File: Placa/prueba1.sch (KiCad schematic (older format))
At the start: 51 parts, among them J1 JACK_2P, U1 MAX232_TID, U2 LM2937, U3 MAX874

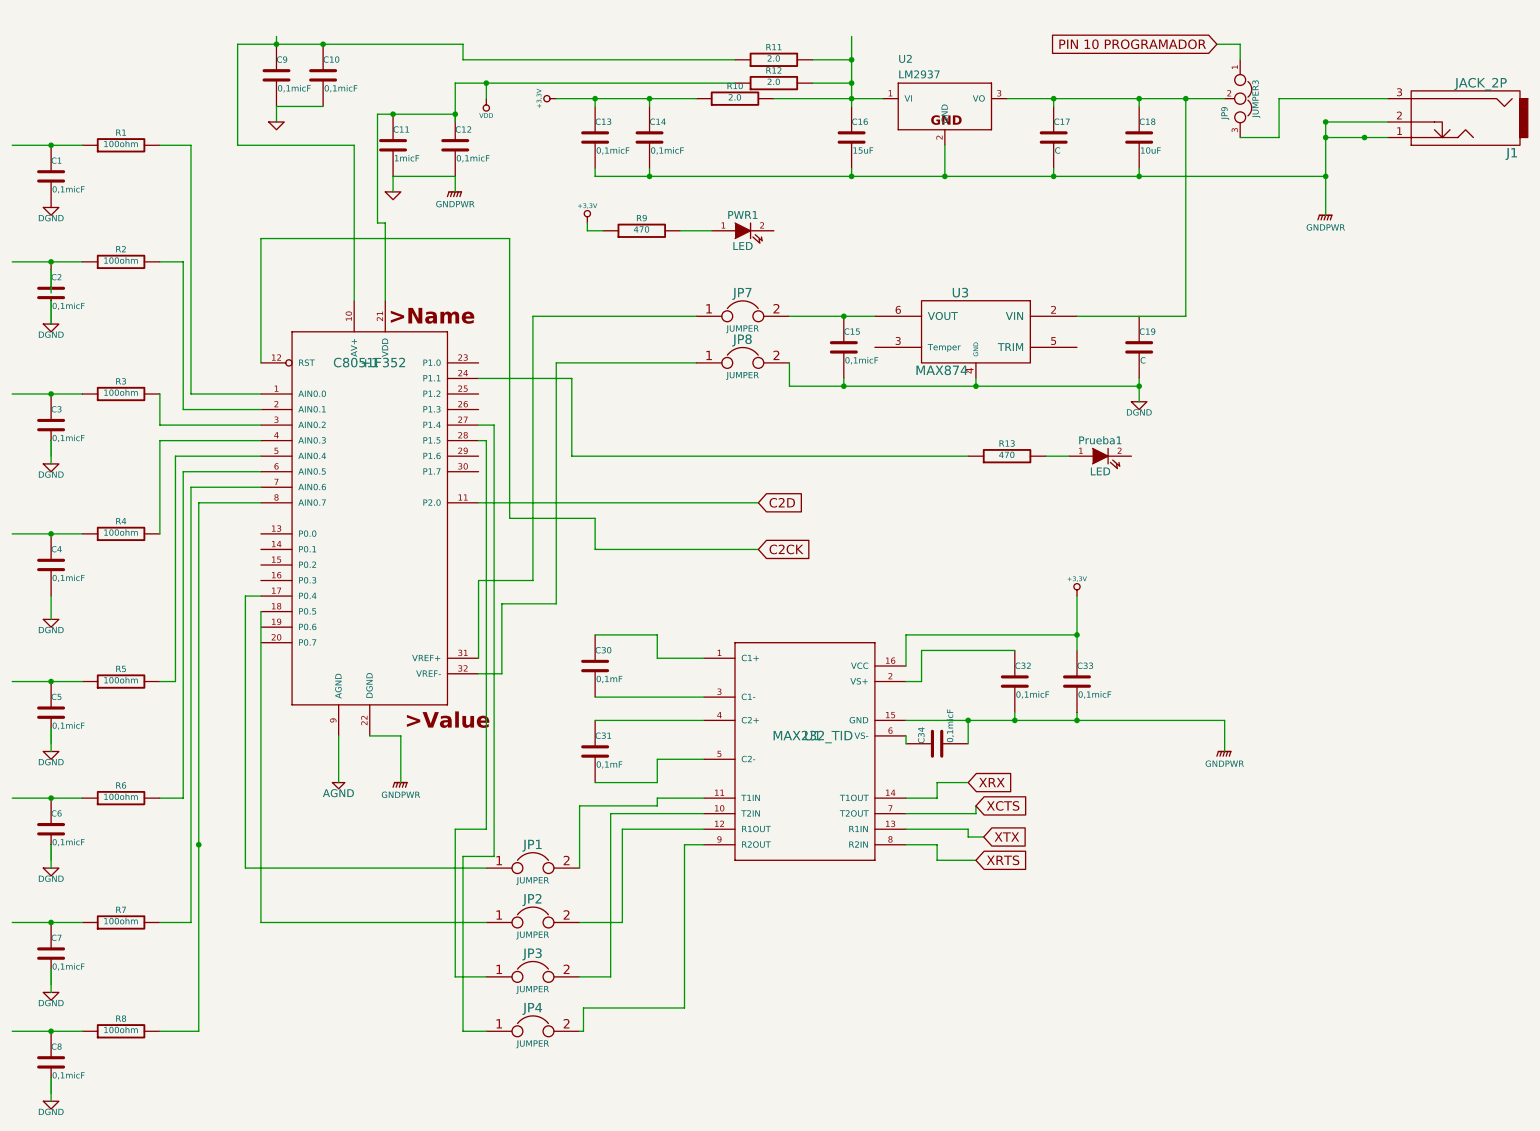
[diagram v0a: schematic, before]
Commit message: Commit Prueba Archivos Placa
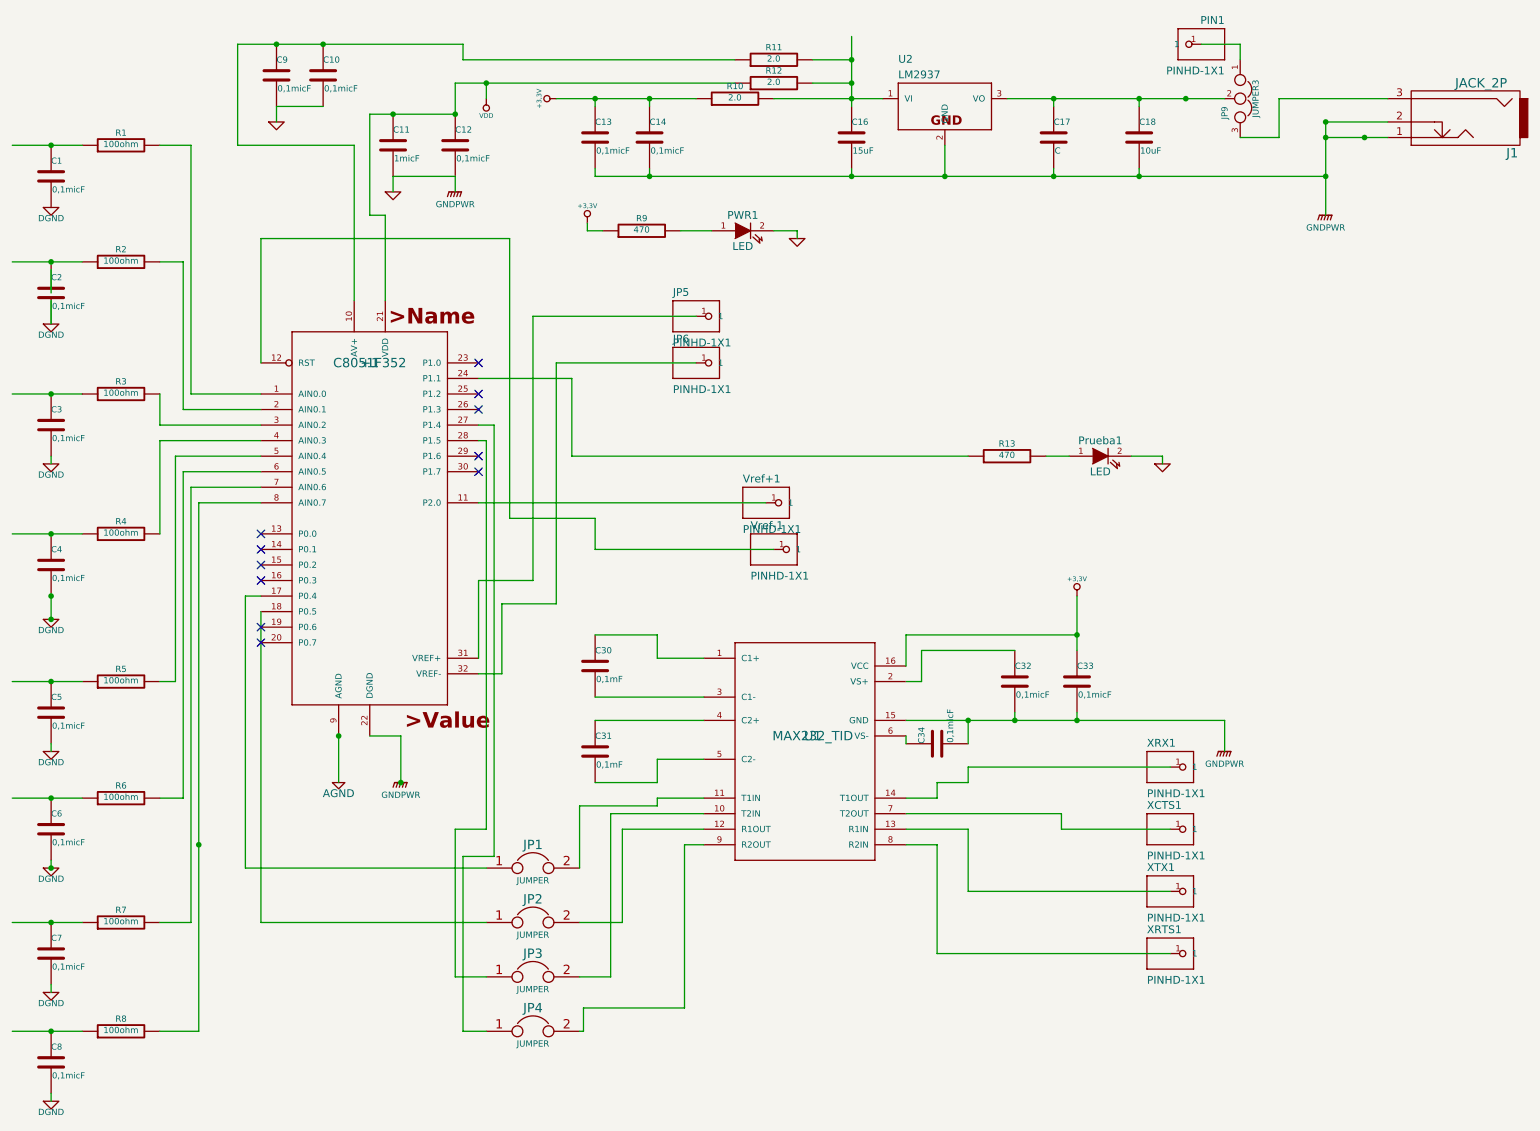
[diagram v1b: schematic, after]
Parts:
- removed C15: 0,1micF, ~, symbol C
- removed C19: C, ~, symbol C
- removed JP7, JP8: JUMPER, ~, symbol JUMPER
- removed U3: MAX874, ~, symbol MAX874
- added JP5, JP6, PIN1, Vref+1, Vref-1, XCTS1, XRTS1, XRX1, XTX1: PINHD-1X1, pinhead-1X01, symbol PINHD-1X1
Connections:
- net labels removed: C2CK, C2D, PIN 10 PROGRAMADOR, XCTS, XRTS, XRX, XTX
- wire segments 177 -> 175
- no-connect marks 0 -> 11

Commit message: Merge remote-tracking branch 'origin/master'
Conflicts:
	.gitignore
	Placa/prueba1.lst
	Source/fuentes/adc
	Source/fuentes/adc.#1
	Source/fuentes/adc.#2
	Source/fuentes/adc.#3
	Source/fuentes/adc.M51
	Source/fuentes/comunicacion.#1
	Source/fuentes/comunicacion.#3
	Source/fuentes/comunicacion.LST
	Source/fuentes/comunicacion.M51
	Source/fuentes/comunicacion.OBJ
	Source/fuentes/configurador.LST
	Source/fuentes/configurador.OBJ
	Source/fuentes/conversor.LST
	Source/fuentes/conversor.OBJ
	Source/fuentes/interfaz.LST
	Source/fuentes/interfaz.OBJ
	Source/fuentes/interrupciones.LST
	Source/fuentes/interrupciones.OBJ
	Source/fuentes/main.LST
	Source/fuentes/main.OBJ
	Source/fuentes/memoria.LST
	Source/fuentes/memoria.OBJ
	Source/test/test_comunicacion.LST
	Source/test/test_comunicacion.OBJ
	Source/test/test_global.LST
	Source/test/test_global.OBJ

commit onda
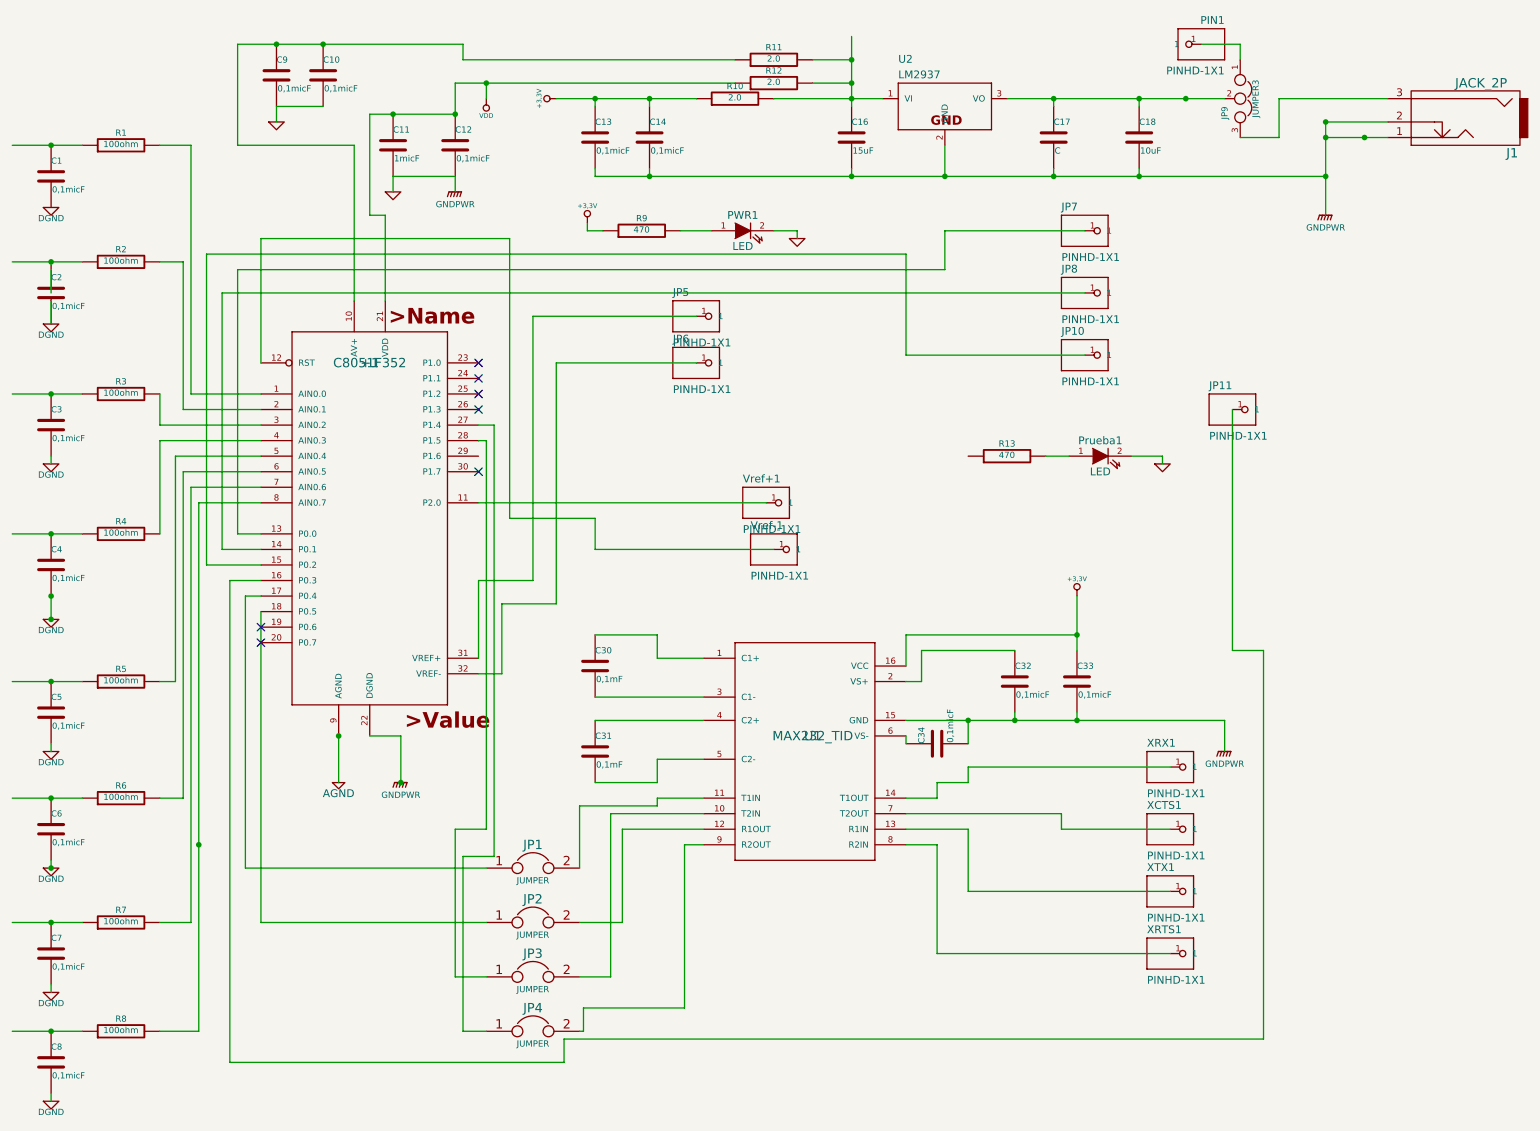
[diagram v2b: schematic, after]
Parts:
- added JP10, JP11, JP7, JP8: PINHD-1X1, pinhead-1X01, symbol PINHD-1X1
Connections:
- wire segments 175 -> 193
- no-connect marks 11 -> 7
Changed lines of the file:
@@
 Sheet 1 1
 Title ""
-Date "4 may 2015"
+Date "8 may 2015"
 Rev ""
 Comp ""
@@
 $EndDescr
 $Comp
-L AGND #PWR10
+L AGND #PWR01
 U 1 1 5524219B
 P 3100 5400
-F 0 "#PWR10" H 3100 5400 40  0001 C CNN
+F 0 "#PWR01" H 3100 5400 40  0001 C CNN
 F 1 "AGND" H 3100 5330 50  0000 C CNN
 F 2 "" H 3100 5400 60  0000 C CNN
@@
 $EndComp
 $Comp
-L DGND #PWR3
+L DGND #PWR02
 U 1 1 552424EC
 P 1250 3350
-F 0 "#PWR3" H 1250 3350 40  0001 C CNN
+F 0 "#PWR02" H 1250 3350 40  0001 C CNN
 F 1 "DGND" H 1250 3280 40  0000 C CNN
 F 2 "" H 1250 3350 60  0000 C CNN
@@
 $EndComp
 $Comp
-L DGND #PWR2
+L DGND #PWR03
 U 1 1 5524256F
 P 1250 2450
-F 0 "#PWR2" H 1250 2450 40  0001 C CNN
+F 0 "#PWR03" H 1250 2450 40  0001 C CNN
 F 1 "DGND" H 1250 2380 40  0000 C CNN
 F 2 "" H 1250 2450 60  0000 C CNN
@@
 $EndComp
 $Comp
-L DGND #PWR1
+L DGND #PWR04
 U 1 1 55242585
 P 1250 1700
-F 0 "#PWR1" H 1250 1700 40  0001 C CNN
+F 0 "#PWR04" H 1250 1700 40  0001 C CNN
 F 1 "DGND" H 1250 1630 40  0000 C CNN
 F 2 "" H 1250 1700 60  0000 C CNN
@@
 $EndComp
 $Comp
-L DGND #PWR4
+L DGND #PWR05
 U 1 1 5524259B
 P 1250 4350
-F 0 "#PWR4" H 1250 4350 40  0001 C CNN
+F 0 "#PWR05" H 1250 4350 40  0001 C CNN
 F 1 "DGND" H 1250 4280 40  0000 C CNN
 F 2 "" H 1250 4350 60  0000 C CNN
@@
 $EndComp
 $Comp
-L DGND #PWR5
+L DGND #PWR06
 U 1 1 552425BD
 P 1250 5200
-F 0 "#PWR5" H 1250 5200 40  0001 C CNN
+F 0 "#PWR06" H 1250 5200 40  0001 C CNN
 F 1 "DGND" H 1250 5130 40  0000 C CNN
 F 2 "" H 1250 5200 60  0000 C CNN
@@
 $EndComp
 $Comp
-L DGND #PWR6
+L DGND #PWR07
 U 1 1 552425D3
 P 1250 5950
-F 0 "#PWR6" H 1250 5950 40  0001 C CNN
+F 0 "#PWR07" H 1250 5950 40  0001 C CNN
 F 1 "DGND" H 1250 5880 40  0000 C CNN
 F 2 "" H 1250 5950 60  0000 C CNN
@@
 $EndComp
 $Comp
-L DGND #PWR7
+L DGND #PWR08
 U 1 1 552426C6
 P 1250 6750
-F 0 "#PWR7" H 1250 6750 40  0001 C CNN
+F 0 "#PWR08" H 1250 6750 40  0001 C CNN
 F 1 "DGND" H 1250 6680 40  0000 C CNN
 F 2 "" H 1250 6750 60  0000 C CNN
@@
 $EndComp
 $Comp
-L DGND #PWR8
+L DGND #PWR09
 U 1 1 552426DB
 P 1250 7450
-F 0 "#PWR8" H 1250 7450 40  0001 C CNN
+F 0 "#PWR09" H 1250 7450 40  0001 C CNN
 F 1 "DGND" H 1250 7380 40  0000 C CNN
 F 2 "" H 1250 7450 60  0000 C CNN
@@
 $EndComp
 $Comp
-L GNDPWR #PWR21
+L GNDPWR #PWR010
 U 1 1 552C3CA0
 P 9450 1750
-F 0 "#PWR21" H 9450 1800 40  0001 C CNN
+F 0 "#PWR010" H 9450 1800 40  0001 C CNN
 F 1 "GNDPWR" H 9450 1670 40  0000 C CNN
 F 2 "" H 9450 1750 60  0000 C CNN
@@
 $EndComp
 $Comp
-L +3,3V #PWR15
+L +3,3V #PWR011
 U 1 1 552C5A6E
 P 4500 1000
-F 0 "#PWR15" H 4500 960 30  0001 C CNN
+F 0 "#PWR011" H 4500 960 30  0001 C CNN
 F 1 "+3,3V" H 4500 1110 30  0000 C CNN
 F 2 "" H 4500 1000 60  0000 C CNN
@@
 $EndComp
 $Comp
-L GNDPWR #PWR13
+L GNDPWR #PWR012
 U 1 1 552C5FBB
 P 3850 1600
-F 0 "#PWR13" H 3850 1650 40  0001 C CNN
+F 0 "#PWR012" H 3850 1650 40  0001 C CNN
 F 1 "GNDPWR" H 3850 1520 40  0000 C CNN
 F 2 "" H 3850 1600 60  0000 C CNN
@@
 $EndComp
 $Comp
-L GND #PWR11
+L GND #PWR013
 U 1 1 552C5FCA
 P 3450 1600
-F 0 "#PWR11" H 3450 1600 30  0001 C CNN
+F 0 "#PWR013" H 3450 1600 30  0001 C CNN
 F 1 "GND" H 3450 1530 30  0001 C CNN
 F 2 "" H 3450 1600 60  0000 C CNN
@@
 $EndComp
 $Comp
-L GND #PWR9
+L GND #PWR014
 U 1 1 552C6618
 P 2700 1150
-F 0 "#PWR9" H 2700 1150 30  0001 C CNN
+F 0 "#PWR014" H 2700 1150 30  0001 C CNN
 F 1 "GND" H 2700 1080 30  0001 C CNN
 F 2 "" H 2700 1150 60  0000 C CNN
@@
 	3500 5100 3500 5400
 $Comp
-L GNDPWR #PWR12
+L GNDPWR #PWR015
 U 1 1 552C76EE
 P 3500 5400
-F 0 "#PWR12" H 3500 5450 40  0001 C CNN
+F 0 "#PWR015" H 3500 5450 40  0001 C CNN
 F 1 "GNDPWR" H 3500 5320 40  0000 C CNN
 F 2 "" H 3500 5400 60  0000 C CNN
@@
 $EndComp
 $Comp
-L GNDPWR #PWR20
+L GNDPWR #PWR016
 U 1 1 552C76FD
 P 8800 5200
-F 0 "#PWR20" H 8800 5250 40  0001 C CNN
+F 0 "#PWR016" H 8800 5250 40  0001 C CNN
 F 1 "GNDPWR" H 8800 5120 40  0000 C CNN
 F 2 "" H 8800 5200 60  0000 C CNN
@@
 $EndComp
 $Comp
-L +3,3V #PWR18
+L +3,3V #PWR017
 U 1 1 552C770C
 P 7850 4200
-F 0 "#PWR18" H 7850 4160 30  0001 C CNN
+F 0 "#PWR017" H 7850 4160 30  0001 C CNN
 F 1 "+3,3V" H 7850 4310 30  0000 C CNN
 F 2 "" H 7850 4200 60  0000 C CNN
@@
 Wire Wire Line
 	1250 4200 1250 4350
-Wire Wire Line
-	4600 2800 4600 3300
-Wire Wire Line
-	4000 2800 4600 2800
-Wire Wire Line
-	4600 3300 7150 3300
-$Comp
-L +3,3V #PWR16
+$Comp
+L +3,3V #PWR018
 U 1 1 55313060
 P 4700 1800
-F 0 "#PWR16" H 4700 1760 30  0001 C CNN
+F 0 "#PWR018" H 4700 1760 30  0001 C CNN
 F 1 "+3,3V" H 4700 1910 30  0000 C CNN
 F 2 "" H 4700 1800 60  0000 C CNN
@@
 NoConn ~ 2600 4400
 NoConn ~ 2600 4500
-NoConn ~ 2600 4100
-NoConn ~ 2600 4000
-NoConn ~ 2600 3900
-NoConn ~ 2600 3800
-NoConn ~ 4000 2700
-NoConn ~ 4000 2900
-NoConn ~ 4000 3000
-NoConn ~ 4000 3300
 NoConn ~ 4000 3400
 Connection ~ 1250 4350
@@
 	3100 5400 3100 5100
 $Comp
-L GND #PWR17
+L GND #PWR019
 U 1 1 553FFE63
 P 6050 1900
-F 0 "#PWR17" H 6050 1900 30  0001 C CNN
+F 0 "#PWR019" H 6050 1900 30  0001 C CNN
 F 1 "GND" H 6050 1830 30  0001 C CNN
 F 2 "" H 6050 1900 60  0000 C CNN
@@
 	6050 1850 6050 1900
 $Comp
-L GND #PWR19
+L GND #PWR020
 U 1 1 553FFF60
 P 8400 3350
-F 0 "#PWR19" H 8400 3350 30  0001 C CNN
+F 0 "#PWR020" H 8400 3350 30  0001 C CNN
 F 1 "GND" H 8400 3280 30  0001 C CNN
 F 2 "" H 8400 3350 60  0000 C CNN
@@
 $EndComp
 $Comp
-L VDD #PWR14
+L VDD #PWR021
 U 1 1 552C5BF6
 P 4050 1000
-F 0 "#PWR14" H 4050 1100 30  0001 C CNN
+F 0 "#PWR021" H 4050 1100 30  0001 C CNN
 F 1 "VDD" H 4050 1110 30  0000 C CNN
 F 2 "" H 4050 1000 60  0000 C CNN
@@
 	1    0    0    -1
 $EndComp
+$Comp
+L PINHD-1X1 JP8
+U 1 1 554D2DF9
+P 8000 2250
+F 0 "JP8" H 7750 2375 50  0000 L BNN
+F 1 "PINHD-1X1" H 7750 2050 50  0000 L BNN
+F 2 "pinhead-1X01" H 8000 2400 50  0001 C CNN
+F 3 "" H 8000 2250 60  0000 C CNN
+	1    8000 2250
+	1    0    0    -1
+$EndComp
+$Comp
+L PINHD-1X1 JP10
+U 1 1 554D2E08
+P 8000 2650
+F 0 "JP10" H 7750 2775 50  0000 L BNN
+F 1 "PINHD-1X1" H 7750 2450 50  0000 L BNN
+F 2 "pinhead-1X01" H 8000 2800 50  0001 C CNN
+F 3 "" H 8000 2650 60  0000 C CNN
+	1    8000 2650
+	1    0    0    -1
+$EndComp
+$Comp
+L PINHD-1X1 JP7
+U 1 1 554D2E17
+P 8000 1850
+F 0 "JP7" H 7750 1975 50  0000 L BNN
+F 1 "PINHD-1X1" H 7750 1650 50  0000 L BNN
+F 2 "pinhead-1X01" H 8000 2000 50  0001 C CNN
+F 3 "" H 8000 1850 60  0000 C CNN
+	1    8000 1850
+	1    0    0    -1
+$EndComp
+$Comp
+L PINHD-1X1 JP11
+U 1 1 554D2E26
+P 8950 3000
+F 0 "JP11" H 8700 3125 50  0000 L BNN
+F 1 "PINHD-1X1" H 8700 2800 50  0000 L BNN
+F 2 "pinhead-1X01" H 8950 3150 50  0001 C CNN
+F 3 "" H 8950 3000 60  0000 C CNN
+	1    8950 3000
+	1    0    0    -1
+$EndComp
+Wire Wire Line
+	7000 1850 7000 2100
+Wire Wire Line
+	7000 1850 7900 1850
+Wire Wire Line
+	2600 3800 2450 3800
+Wire Wire Line
+	2450 3800 2450 2100
+Wire Wire Line
+	2450 2100 7000 2100
+Wire Wire Line
+	7900 2250 2350 2250
+Wire Wire Line
+	2350 2250 2350 3900
+Wire Wire Line
+	2350 3900 2600 3900
+Wire Wire Line
+	2600 4000 2250 4000
+Wire Wire Line
+	2250 4000 2250 2000
+Wire Wire Line
+	2250 2000 6750 2000
+Wire Wire Line
+	6750 2000 6750 2650
+Wire Wire Line
+	6750 2650 7900 2650
+Wire Wire Line
+	8850 3000 8850 4550
+Wire Wire Line
+	8850 4550 9050 4550
+Wire Wire Line
+	9050 4550 9050 7050
+Wire Wire Line
+	9050 7050 4550 7050
+Wire Wire Line
+	4550 7050 4550 7200
+Wire Wire Line
+	4550 7200 2400 7200
+Wire Wire Line
+	2400 7200 2400 4100
+Wire Wire Line
+	2400 4100 2600 4100
+NoConn ~ 4000 2700
+NoConn ~ 4000 2800
+NoConn ~ 4000 2900
+NoConn ~ 4000 3000
 $EndSCHEMATC
